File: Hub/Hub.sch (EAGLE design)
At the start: 32 parts

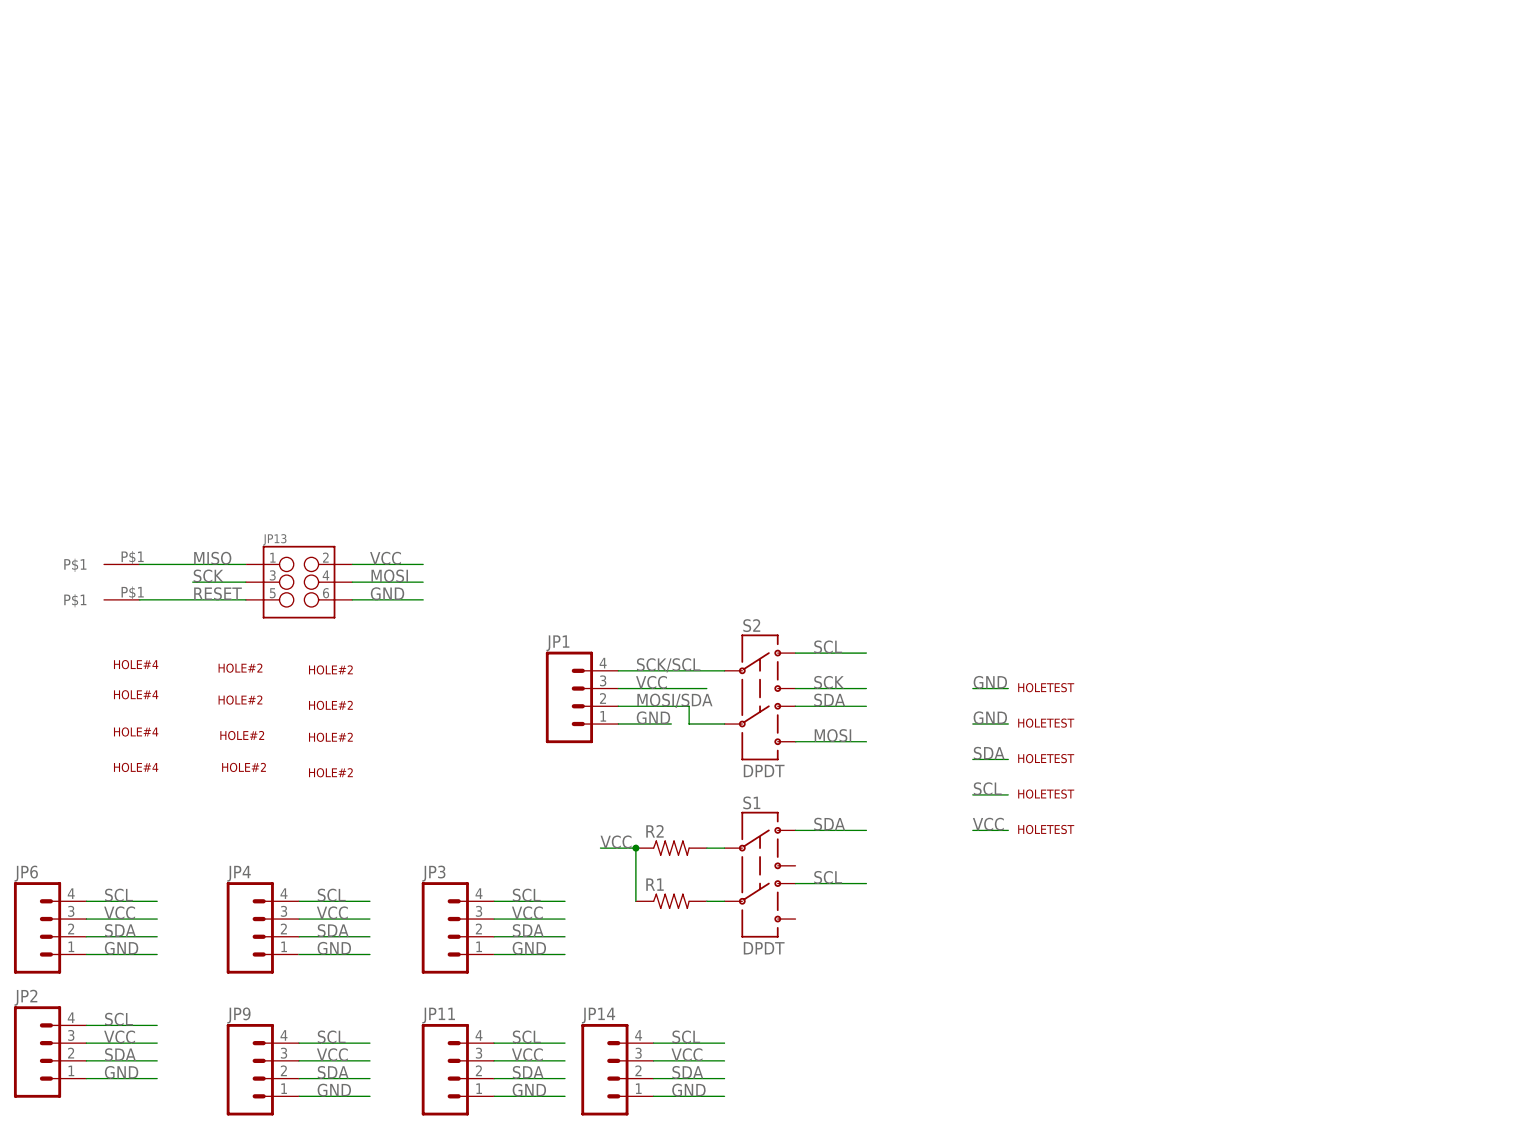
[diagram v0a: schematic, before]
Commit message: Latest version of schematics and boards
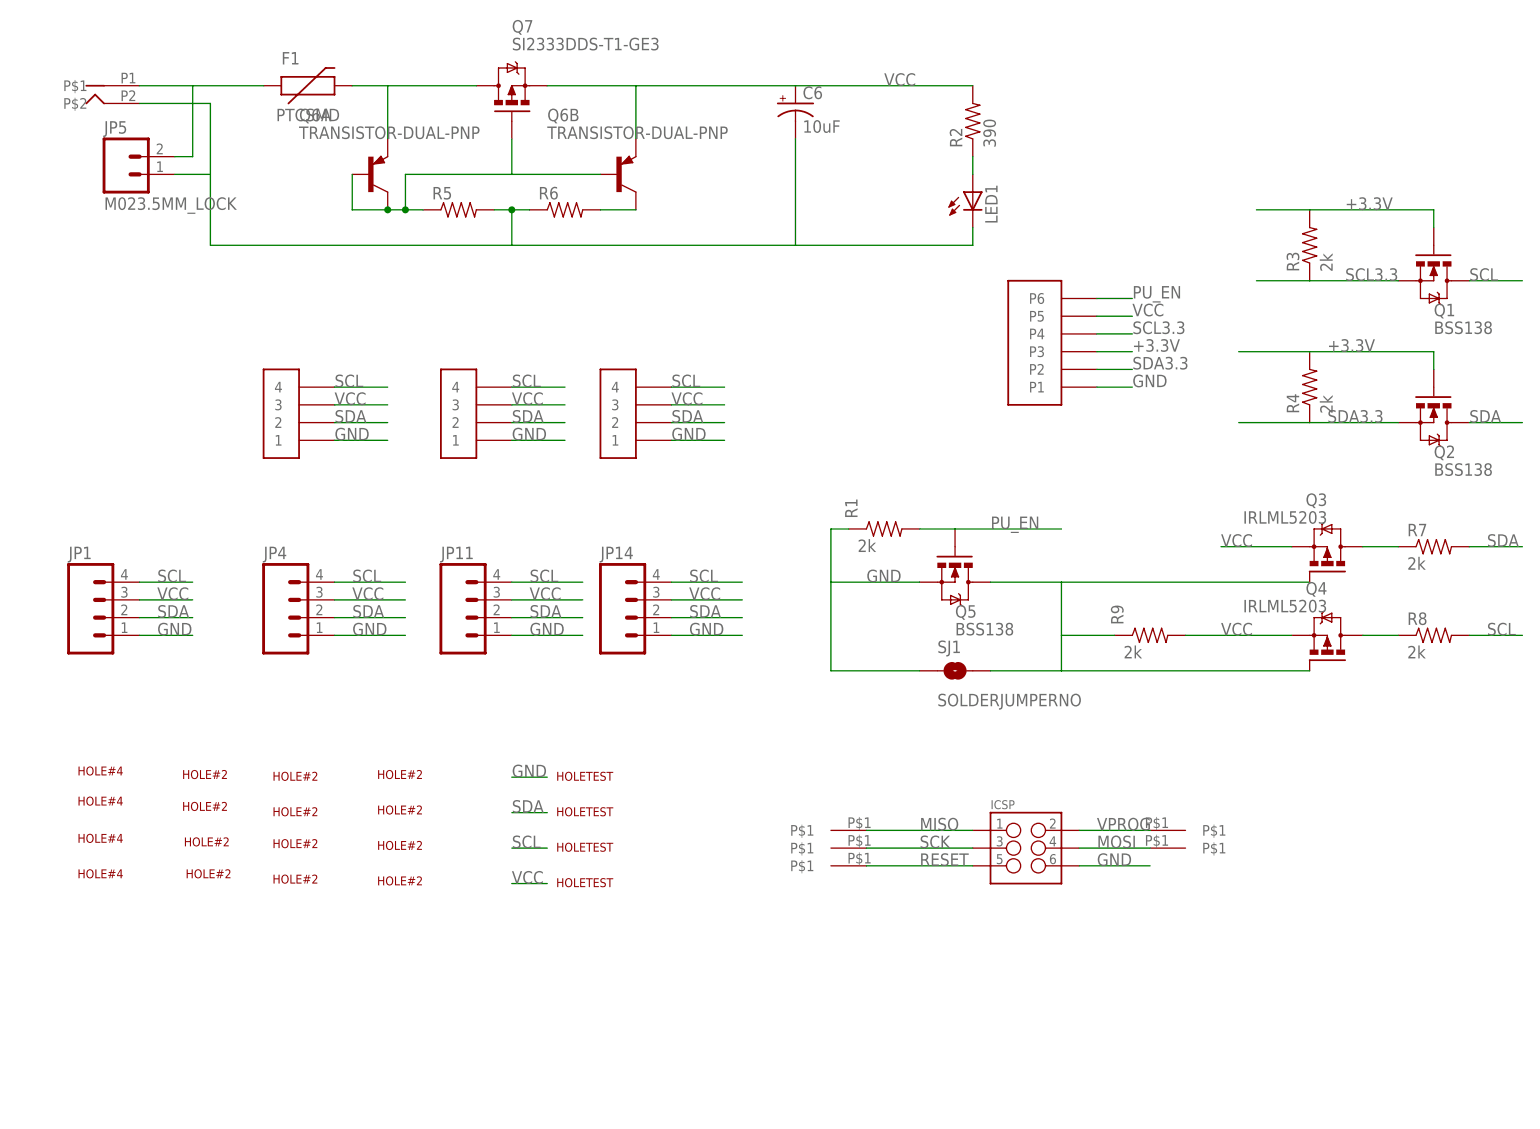
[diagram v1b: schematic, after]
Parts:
- removed JP13: (no value), SparkFun-Connectors:M03X2SHROUD
- removed JP9: (no value), SparkFun-Connectors:M04POLAR_LOCK
- removed S1, S2: DPDT, SparkFun-Electromechanical:SWITCH-DPDTAYZ0202
- added C6: 10uF, SparkFun-Capacitors:10UF-20V-10%(TANT)
- added F1: PTCSMD, SparkFun-PowerIC:PTCSMD
- added ICSP: (no value), SparkFun-Connectors:M03X22X3_SILK_SM
- added JP5: M023.5MM_LOCK, SparkFun-Connectors:M023.5MM_LOCK
- added LED1: (no value), led:LEDCHIPLED_0805
- added Q1, Q2, Q5: BSS138, SparkFun-DiscreteSemi:MOSFET-NCHANNELBSS138
- added Q3, Q4: IRLML5203, transistor-power:IRLML5203
- added Q6: TRANSISTOR-DUAL-PNP, IntegerLabs:TRANSISTOR-DUAL-PNP
- added Q7: SI2333DDS-T1-GE3, SparkFun-DiscreteSemi:MOSFET-PCHANNELSMD
- added R3, R4: 2k, SparkFun-Passives:RESISTOR0805-RES
- added R5, R6: (no value), SparkFun-Resistors:RESISTOR0805-RES
- added R7, R8, R9: 2k, SparkFun-Resistors:RESISTOR0805-RES
- added SJ1: SOLDERJUMPERNO, SparkFun-Passives:SOLDERJUMPERNO
- added U$21: DC-JACK, IntegerLabs:DC-JACK
- added U$22, U$23, U$24: SPRING-CONNECTOR, IntegerLabs:SPRING-CONNECTOR
- added U$25, U$26, U$27: HOLE#2, IntegerLabs:HOLE#2
- added U$28: HEADER-1X6MOLEX-KK254, IntegerLabs:HEADER-1X6MOLEX-KK254
- JP2, JP3, JP6: value (none) -> HEADER-1X4MOLEX-SL; device SparkFun-Connectors:M04POLAR_LOCK -> IntegerLabs:HEADER-1X4MOLEX-SL
- R1: value (none) -> 2k
- R2: value (none) -> 390; device SparkFun-Resistors:RESISTOR0805-RES -> SparkFun-Passives:RESISTOR0805-RES
- U$15: value HOLETEST -> HOLE#2; device IntegerLabs:HOLETEST -> IntegerLabs:HOLE#2
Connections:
- removed net MOSI/SDA: JP1.2, S2.5
- removed net SCK/SCL: JP1.4, S2.2
- new net +3.3V: Q1.G, Q2.G, R3.2, R4.2, U$28.P3
- new net N$1: Q3.G, Q4.G, Q5.D, R9.1, SJ1.2
- new net N$2: F1.1, JP5.2, U$21.P$1
- new net N$5: F1.2, Q6A.E, Q7.D
- new net N$6: Q3.D, R7.1
- new net N$7: Q4.D, R8.1
- new net N$8: LED1.A, R2.1
- new net PU_EN: Q5.G, R1.2, U$28.P6
- new net SCL3.3: Q1.S, R3.1, U$28.P4
- new net SDA3.3: Q2.S, R4.1, U$28.P2
- new net VPROG: ICSP.2, U$24.P$1
- net GND: now also C6.-, ICSP.6, JP5.1, LED1.C, Q5.S, R1.1, R5.2, R6.1, SJ1.1, U$21.P$2, U$28.P1; no longer JP13.6, JP9.1, U$15.HOLE
- net MISO: now also ICSP.1; no longer JP13.1
- net MOSI: now also ICSP.4, U$23.P$1; no longer JP13.4, S2.6
- net N$3: now also Q6A.B, Q6A.C, Q6B.B, Q7.G, R5.1; no longer R1.2, S1.5
- net N$4: now also Q6B.C, R6.2; no longer R2.2, S1.2
- net RESET: now also ICSP.5; no longer JP13.5
- net SCK: now also ICSP.3, U$22.P$1; no longer JP13.3, S2.3
- net SCL: now also JP1.4, Q1.D, R8.2; no longer JP9.4, S1.4, S2.1
- net SDA: now also JP1.2, Q2.D, R7.2; no longer JP9.2, S1.1, S2.4
- net VCC: now also C6.+, Q3.S, Q4.S, Q6B.E, Q7.S, R2.2, R9.2, U$28.P5; no longer JP13.2, JP9.3, R1.1, R2.1
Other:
- moved on the sheet: JP1, JP11, JP14, JP4, R1, R2
